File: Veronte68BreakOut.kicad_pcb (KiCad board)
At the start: 2 copper layers, 11 parts, among them J1 DC37_Receptacle_MountingHoles, J10 Barrel_Jack_Switch, J11 Barrel_Jack_Switch, J2 DC37_Receptacle_MountingHoles, J3 DE9_Receptacle_MountingHoles, J4 Conn_01x19, J5 Conn_01x11, J6 Conn_01x19, J7 Conn_01x11, J8 Conn_01x05, J9 Conn_01x03

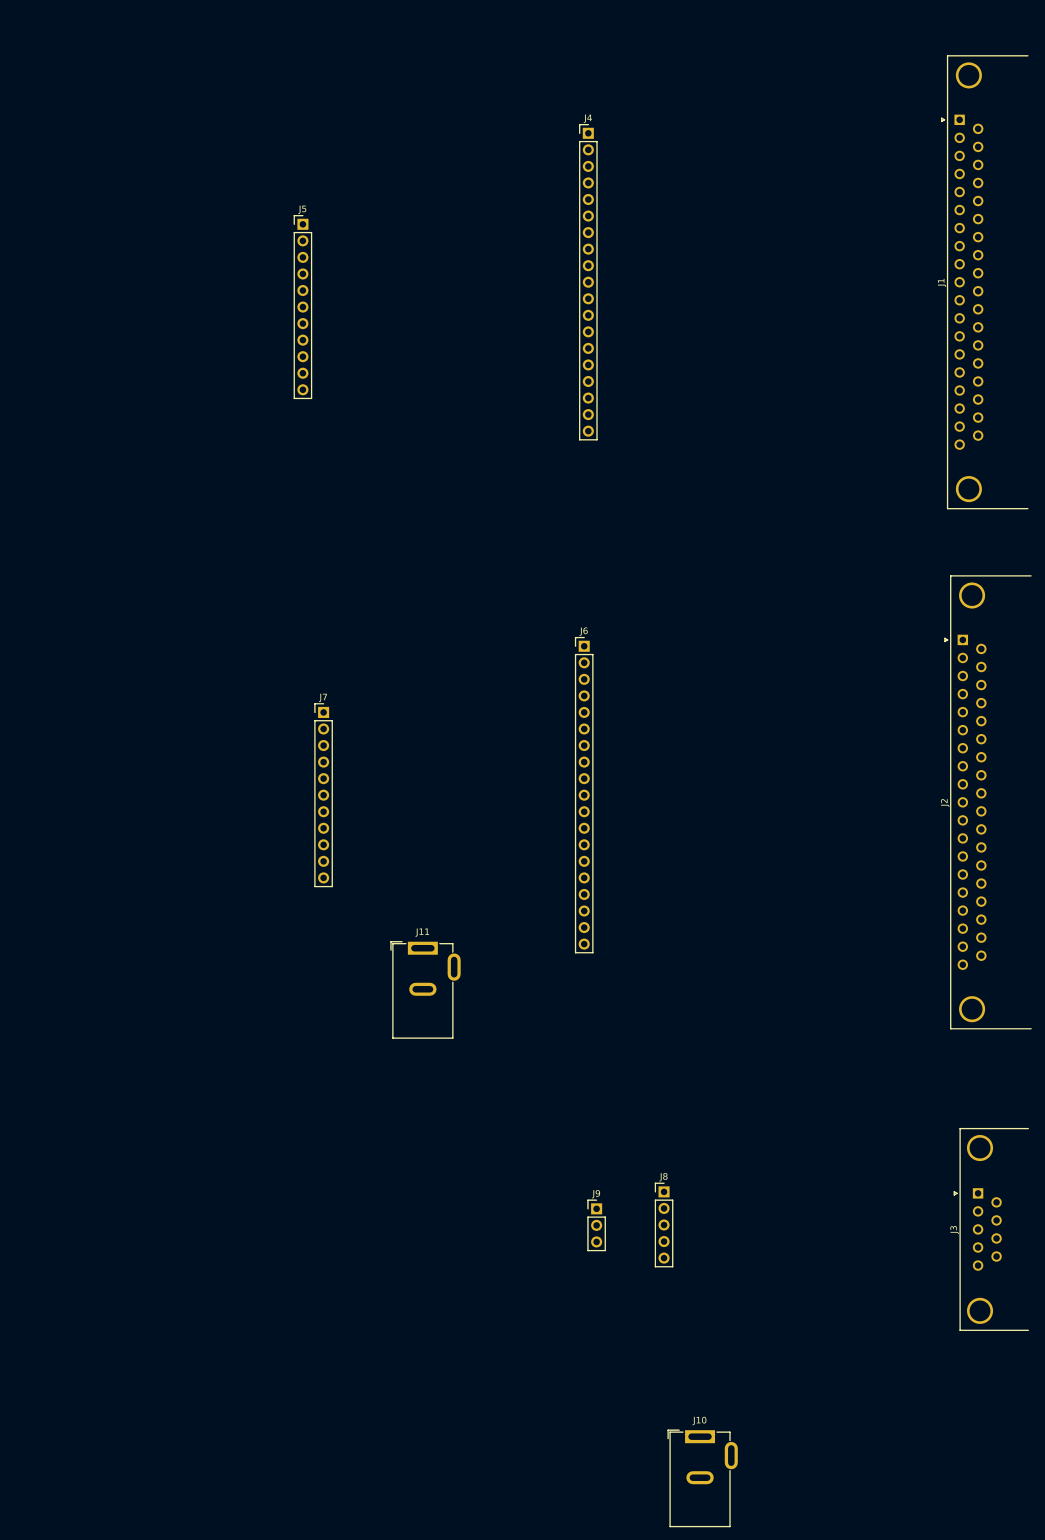
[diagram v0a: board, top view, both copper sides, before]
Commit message: pcbを作成
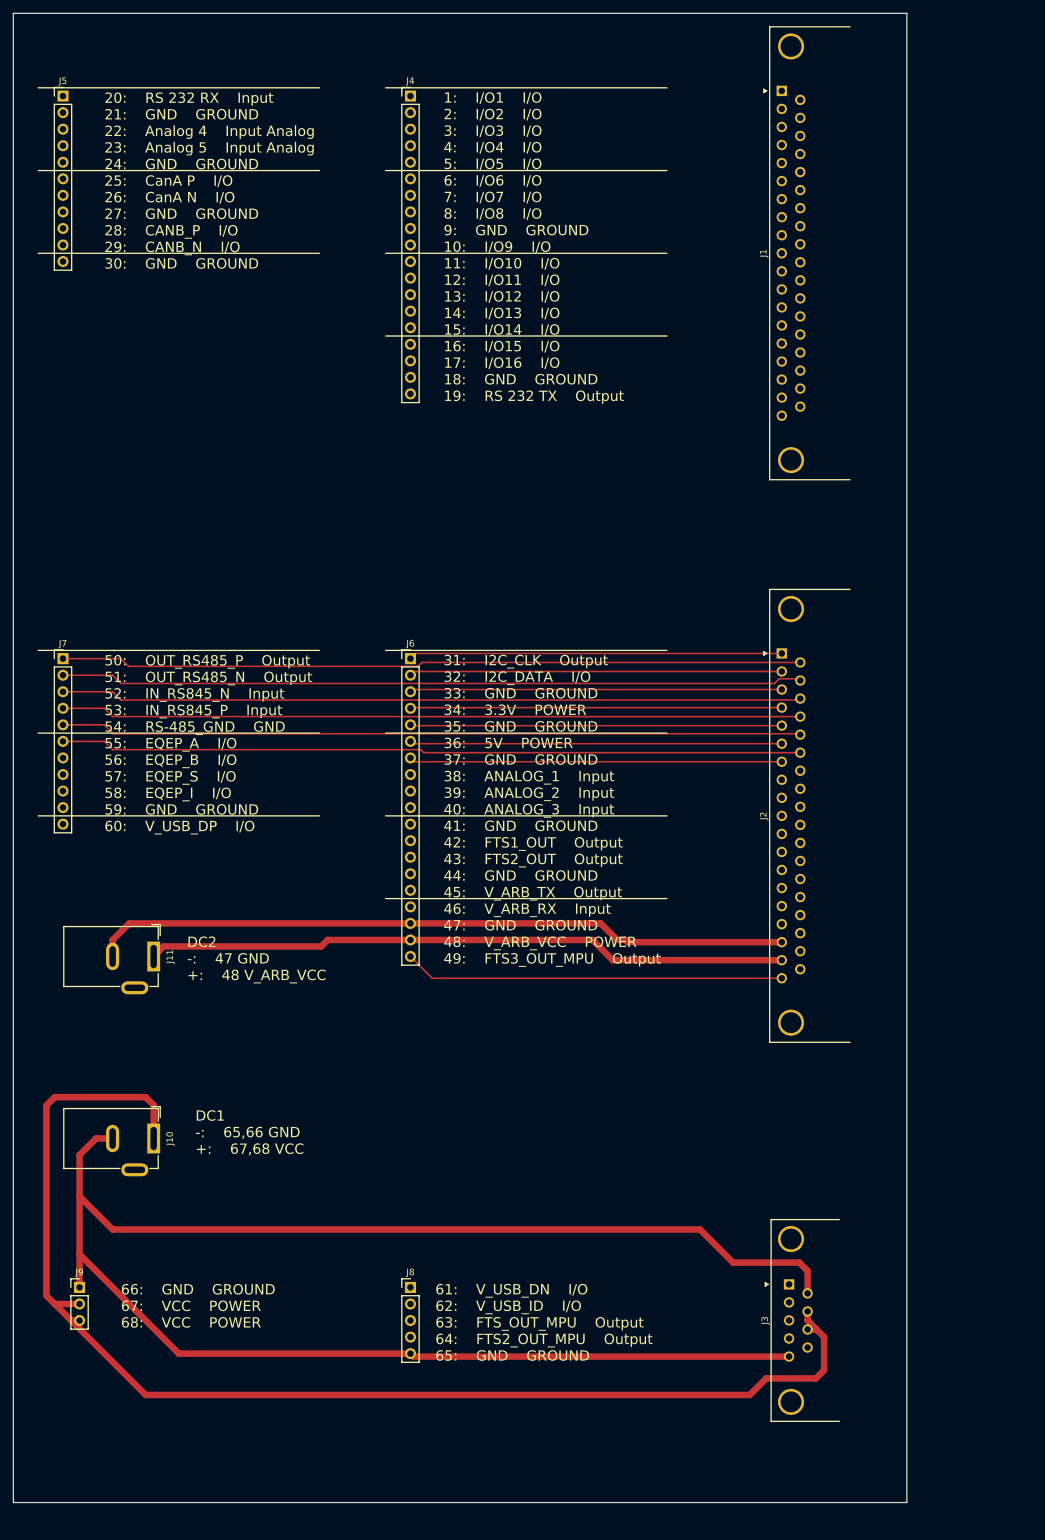
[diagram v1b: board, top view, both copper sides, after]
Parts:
- moved J10 95.5 mm to (87.6, 198.1), turned to -90 degrees
- moved J9 80.3 mm to (76.2, 221.0)
- moved J5 41.8 mm to (73.7, 38.1)
- moved J8 41.6 mm to (127.0, 221.0)
- moved J11 41.3 mm to (87.6, 170.2), turned to -90 degrees
- moved J7 40.8 mm to (73.7, 124.5)
- moved J3 32.2 mm to (185.1, 220.5)
- moved J4 27.9 mm to (127.0, 38.1)
- moved J2 27.9 mm to (184.0, 123.7)
- moved J1 27.7 mm to (184.0, 37.3)
- moved J6 26.7 mm to (127.0, 124.5)
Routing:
- net Net-(J8-Pin_5): track 0.00 -> 261.8 mm
- net Net-(J9-Pin_2): track 0.00 -> 195.6 mm
- net Net-(J7-Pin_2): track 0.00 -> 114.1 mm
- net Net-(J7-Pin_1): track 0.00 -> 113.9 mm
- net Net-(J7-Pin_6): track 0.00 -> 113.9 mm
- net Net-(J7-Pin_5): track 0.00 -> 113.8 mm
- net Net-(J7-Pin_3): track 0.00 -> 113.8 mm
- net Net-(J7-Pin_4): track 0.00 -> 113.7 mm
- net Net-(J6-Pin_17): track 0.00 -> 107.5 mm
- net Net-(J6-Pin_18): track 0.00 -> 98.8 mm
- net Net-(J6-Pin_19): track 0.00 -> 58.4 mm
- net Net-(J6-Pin_1): track 0.00 -> 57.3 mm
- net Net-(J6-Pin_7): track 0.00 -> 57.2 mm
- net Net-(J6-Pin_2): track 0.00 -> 57.2 mm
- net Net-(J6-Pin_6): track 0.00 -> 57.1 mm
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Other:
- board outline added: 137.2 x 228.6 mm
- board text added: "1: I/O1 I/O 2: I/O2 I/O 3: I/O3 I/O 4: I/O4 I/O 5: I/O5 I/O 6: I/O6 I/O 7: I/O7 I/O 8: I/O8 I/O 9: GND GROUND 10: I/O9 I/O 11: I/O10 I/O 12: I/O11 I/O 13: I/O12 I/O 14: I/O13 I/O 15: I/O14 I/O 16: I/O15 I/O 17: I/O16 I/O 18: GND GROUND 19: RS 232 TX Output"
- board text added: "20: RS 232 RX Input 21: GND GROUND 22: Analog 4 Input Analog 23: Analog 5 Input Analog 24: GND GROUND 25: CanA P I/O 26: CanA N I/O 27: GND GROUND 28: CANB_P I/O 29: CANB_N I/O 30: GND GROUND"
- board text added: "31: I2C_CLK Output 32: I2C_DATA I/O 33: GND GROUND 34: 3.3V POWER 35: GND GROUND 36: 5V POWER 37: GND GROUND 38: ANALOG_1 Input 39: ANALOG_2 Input 40: ANALOG_3 Input 41: GND GROUND 42: FTS1_OUT Output 43: FTS2_OUT Output 44: GND GROUND 45: V_ARB_TX Output 46: V_ARB_RX Input 47: GND GROUND 48: V_ARB_VCC POWER 49: FTS3_OUT_MPU Output"
- board text added: "50: OUT_RS485_P Output 51: OUT_RS485_N Output 52: IN_RS845_N Input 53: IN_RS845_P Input 54: RS-485_GND GND 55: EQEP_A I/O 56: EQEP_B I/O 57: EQEP_S I/O 58: EQEP_I I/O 59: GND GROUND 60: V_USB_DP I/O"
- board text added: "61: V_USB_DN I/O 62: V_USB_ID I/O 63: FTS_OUT_MPU Output 64: FTS2_OUT_MPU Output 65: GND GROUND"
- board text added: "66: GND GROUND 67: VCC POWER 68: VCC POWER"
- board text added: "DC1 -: 65,66 GND +: 67,68 VCC"
- board text added: "DC2 -: 47 GND +: 48 V_ARB_VCC"

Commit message: rooting finish
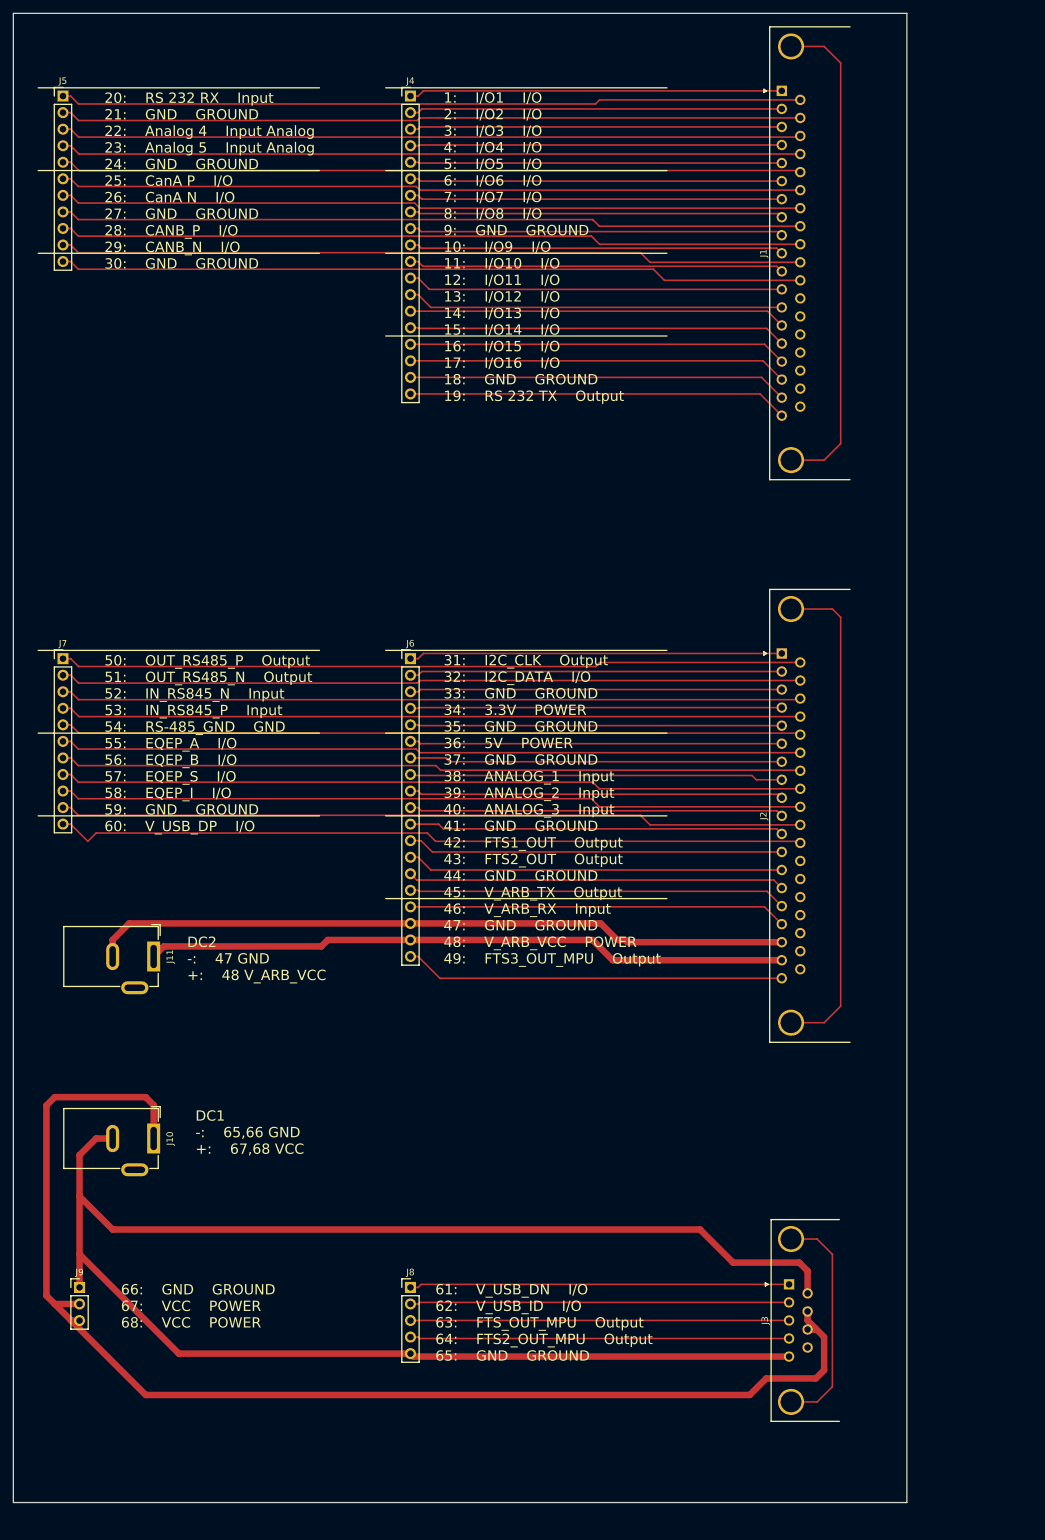
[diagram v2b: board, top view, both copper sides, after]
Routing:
- net Net-(J7-Pin_11): track 0.00 -> 115.4 mm
- net Net-(J5-Pin_11): track 0.00 -> 114.4 mm
- net Net-(J7-Pin_10): track 0.00 -> 114.3 mm
- net Net-(J5-Pin_10): track 0.00 -> 114.3 mm
- net Net-(J7-Pin_9): track 0.00 -> 114.2 mm
- net Net-(J5-Pin_9): track 0.00 -> 114.2 mm
- net Net-(J7-Pin_8): track 0.00 -> 114.1 mm
- net Net-(J5-Pin_8): track 0.00 -> 114.1 mm
- net Net-(J7-Pin_7): track 0.00 -> 114.0 mm
- net Net-(J5-Pin_7): track 0.00 -> 114.0 mm
- net Net-(J5-Pin_1): track 0.00 -> 113.9 mm
- net Net-(J5-Pin_6): track 0.00 -> 113.9 mm
- net Net-(J5-Pin_2): track 0.00 -> 113.8 mm
- net Net-(J5-Pin_5): track 0.00 -> 113.8 mm
- net Net-(J5-Pin_3): track 0.00 -> 113.8 mm
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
